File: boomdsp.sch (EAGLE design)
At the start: 23 parts

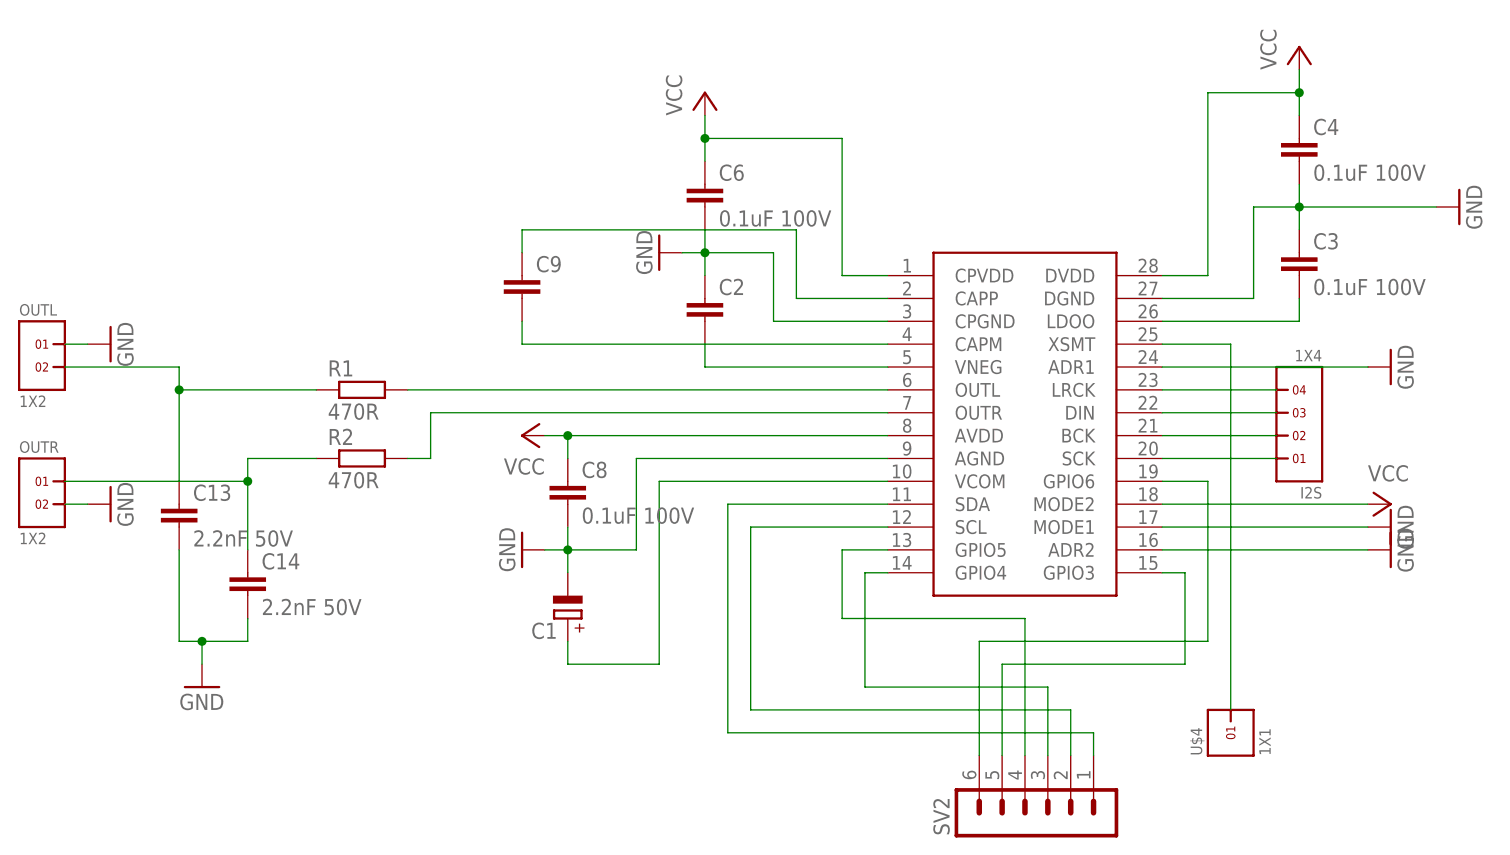
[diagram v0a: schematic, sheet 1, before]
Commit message: final prototype
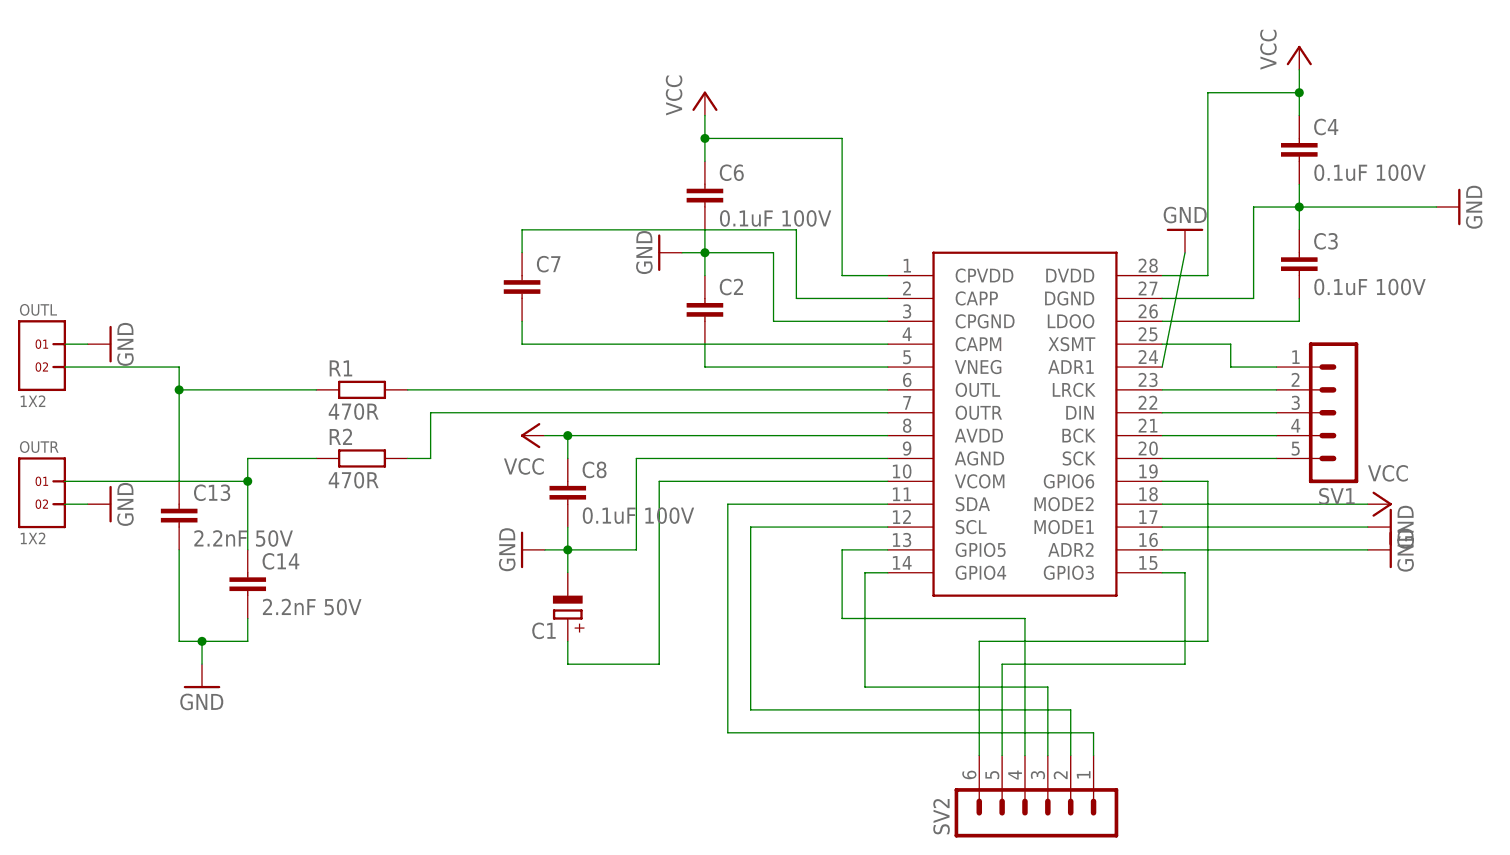
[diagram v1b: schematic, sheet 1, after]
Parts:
- removed C9: (no value), rcl:C-EUC1206
- removed I2S: 1X4, headers(2mm):1X4
- removed U$4: 1X1, headers(2mm):1X1
- added C7: (no value), resistor:C-EUC0805
- added SV1: (no value), con-lstb:MA05-1
- C2: device rcl:C-EUC1206 -> resistor:C-EUC0805
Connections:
- removed net N$18: U$1.MODE1
- net GND: now also U$1.MODE1
- net N$12: now also C7.1; no longer C9.1
- net N$13: now also SV1.2; no longer I2S.4
- net N$14: now also SV1.3; no longer I2S.3
- net N$16: now also SV1.4; no longer I2S.2
- net N$17: now also SV1.5; no longer I2S.1
- net N$21: now also SV1.1; no longer U$4.1
- net N$5: now also C7.2; no longer C9.2
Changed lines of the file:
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@@
 <?xml version="1.0" encoding="utf-8"?>
 <!DOCTYPE eagle SYSTEM "eagle.dtd">
-<eagle version="8.1.0">
+<eagle version="7.6.0">
 <drawing>
 <settings>
@@
 <part name="P+2" library="supply1" deviceset="VCC" device=""/>
 <part name="U$1" library="boomdsp" deviceset="PCM5142_I2C" device=""/>
-<part name="I2S" library="headers(2mm)" deviceset="1X4" device=""/>
 <part name="GND3" library="supply1" deviceset="GND" device=""/>
 <part name="POWER" library="headers(2mm)" deviceset="1X2" device=""/>
@@
 <part name="GND11" library="supply1" deviceset="GND" device=""/>
 <part name="C1" library="rcl" deviceset="CPOL-EU" device="E3.5-8"/>
-<part name="U$4" library="headers(2mm)" deviceset="1X1" device=""/>
 <part name="P+5" library="supply1" deviceset="VCC" device=""/>
 <part name="P+6" library="supply1" deviceset="VCC" device=""/>
@@
 <part name="H3" library="holes" deviceset="MOUNT-HOLE" device="3.2"/>
 <part name="H4" library="holes" deviceset="MOUNT-HOLE" device="3.2"/>
-<part name="C9" library="rcl" deviceset="C-EU" device="C1206"/>
-<part name="C2" library="rcl" deviceset="C-EU" device="C1206"/>
+<part name="C7" library="resistor" deviceset="C-EU" device="C0805"/>
+<part name="C2" library="resistor" deviceset="C-EU" device="C0805"/>
+<part name="SV1" library="con-lstb" deviceset="MA05-1" device=""/>
 </parts>
 <sheets>
@@
 <instance part="P+2" gate="VCC" x="35.56" y="93.98"/>
 <instance part="U$1" gate="G$1" x="71.12" y="58.42"/>
-<instance part="I2S" gate="G$1" x="101.6" y="58.42" rot="R180"/>
 <instance part="GND3" gate="1" x="111.76" y="45.72" rot="R90"/>
 <instance part="GND5" gate="1" x="15.24" y="43.18" rot="R270"/>
@@
 <instance part="P+4" gate="VCC" x="111.76" y="48.26" rot="R270"/>
 <instance part="GND10" gate="1" x="111.76" y="43.18" rot="R90"/>
-<instance part="GND11" gate="1" x="111.76" y="63.5" rot="R90"/>
+<instance part="GND11" gate="1" x="88.9" y="78.74" rot="R180"/>
 <instance part="C1" gate="G$1" x="20.32" y="35.56" rot="R180"/>
-<instance part="U$4" gate="G$1" x="93.98" y="22.86" rot="R90"/>
 <instance part="SV2" gate="1" x="71.12" y="12.7" rot="R90"/>
-<instance part="C9" gate="G$1" x="15.24" y="73.66"/>
+<instance part="C7" gate="G$1" x="15.24" y="73.66"/>
 <instance part="C2" gate="G$1" x="35.56" y="71.12"/>
+<instance part="SV1" gate="G$1" x="106.68" y="58.42" rot="R180"/>
 </instances>
 <busses>
@@
 <wire x1="15.24" y1="66.04" x2="15.24" y2="68.58" width="0.1524" layer="91"/>
 <pinref part="U$1" gate="G$1" pin="CAPM"/>
-<pinref part="C9" gate="G$1" pin="2"/>
+<pinref part="C7" gate="G$1" pin="2"/>
 </segment>
 </net>
@@
 <wire x1="15.24" y1="78.74" x2="15.24" y2="76.2" width="0.1524" layer="91"/>
 <pinref part="U$1" gate="G$1" pin="CAPP"/>
-<pinref part="C9" gate="G$1" pin="1"/>
+<pinref part="C7" gate="G$1" pin="1"/>
 </segment>
 </net>
@@
 <pinref part="U$1" gate="G$1" pin="ADR1"/>
 <pinref part="GND11" gate="1" pin="GND"/>
-<wire x1="86.36" y1="63.5" x2="109.22" y2="63.5" width="0.1524" layer="91"/>
+<wire x1="86.36" y1="63.5" x2="88.9" y2="76.2" width="0.1524" layer="91"/>
 </segment>
 <segment>
@@
 <pinref part="U$1" gate="G$1" pin="ADR2"/>
 <wire x1="109.22" y1="43.18" x2="86.36" y2="43.18" width="0.1524" layer="91"/>
+</segment>
+<segment>
+<pinref part="U$1" gate="G$1" pin="MODE1"/>
+<pinref part="GND3" gate="1" pin="GND"/>
+<wire x1="86.36" y1="45.72" x2="109.22" y2="45.72" width="0.1524" layer="91"/>
 </segment>
 </net>
@@
 <segment>
 <pinref part="U$1" gate="G$1" pin="LRCK"/>
-<pinref part="I2S" gate="G$1" pin="4"/>
 <wire x1="86.36" y1="60.96" x2="99.06" y2="60.96" width="0.1524" layer="91"/>
+<pinref part="SV1" gate="G$1" pin="2"/>
 </segment>
 </net>
@@
 <segment>
 <pinref part="U$1" gate="G$1" pin="DIN"/>
-<pinref part="I2S" gate="G$1" pin="3"/>
 <wire x1="86.36" y1="58.42" x2="99.06" y2="58.42" width="0.1524" layer="91"/>
+<pinref part="SV1" gate="G$1" pin="3"/>
 </segment>
 </net>
@@
 <segment>
 <pinref part="U$1" gate="G$1" pin="BCK"/>
-<pinref part="I2S" gate="G$1" pin="2"/>
 <wire x1="86.36" y1="55.88" x2="99.06" y2="55.88" width="0.1524" layer="91"/>
+<pinref part="SV1" gate="G$1" pin="4"/>
 </segment>
 </net>
@@
 <segment>
 <pinref part="U$1" gate="G$1" pin="SCK"/>
-<pinref part="I2S" gate="G$1" pin="1"/>
 <wire x1="86.36" y1="53.34" x2="99.06" y2="53.34" width="0.1524" layer="91"/>
-</segment>
-</net>
-<net name="N$18" class="0">
-<segment>
-<pinref part="U$1" gate="G$1" pin="MODE1"/>
-<wire x1="86.36" y1="45.72" x2="109.22" y2="45.72" width="0.1524" layer="91"/>
-<pinref part="GND3" gate="1" pin="GND"/>
+<pinref part="SV1" gate="G$1" pin="5"/>
 </segment>
 </net>
@@
 <pinref part="U$1" gate="G$1" pin="XSMT"/>
 <wire x1="86.36" y1="66.04" x2="93.98" y2="66.04" width="0.1524" layer="91"/>
-<wire x1="93.98" y1="66.04" x2="93.98" y2="25.4" width="0.1524" layer="91"/>
-<pinref part="U$4" gate="G$1" pin="1"/>
-</segment>
-</net>
+<wire x1="93.98" y1="66.04" x2="93.98" y2="63.5" width="0.1524" layer="91"/>
+<pinref part="SV1" gate="G$1" pin="1"/>
+<wire x1="93.98" y1="63.5" x2="99.06" y2="63.5" width="0.1524" layer="91"/>
+</segment>
+</net>
